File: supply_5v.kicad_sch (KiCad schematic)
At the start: 13 parts, among them IC2 TPS564242DRLR

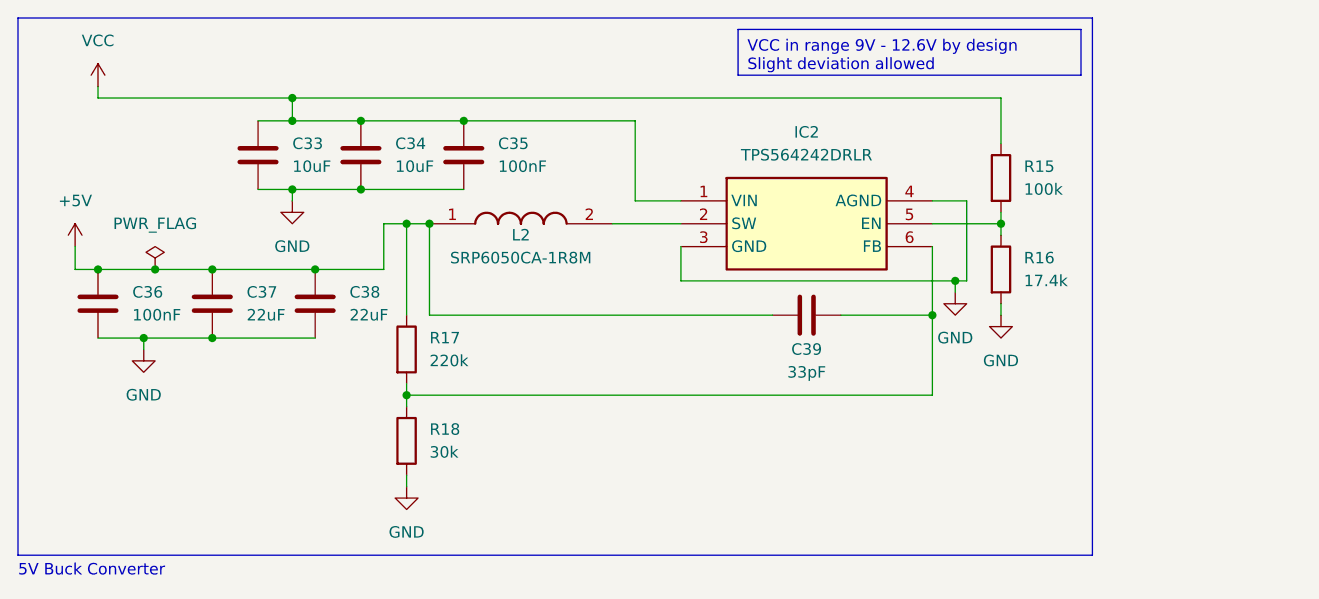
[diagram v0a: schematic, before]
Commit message: Uploaded all project files, finished PCB design
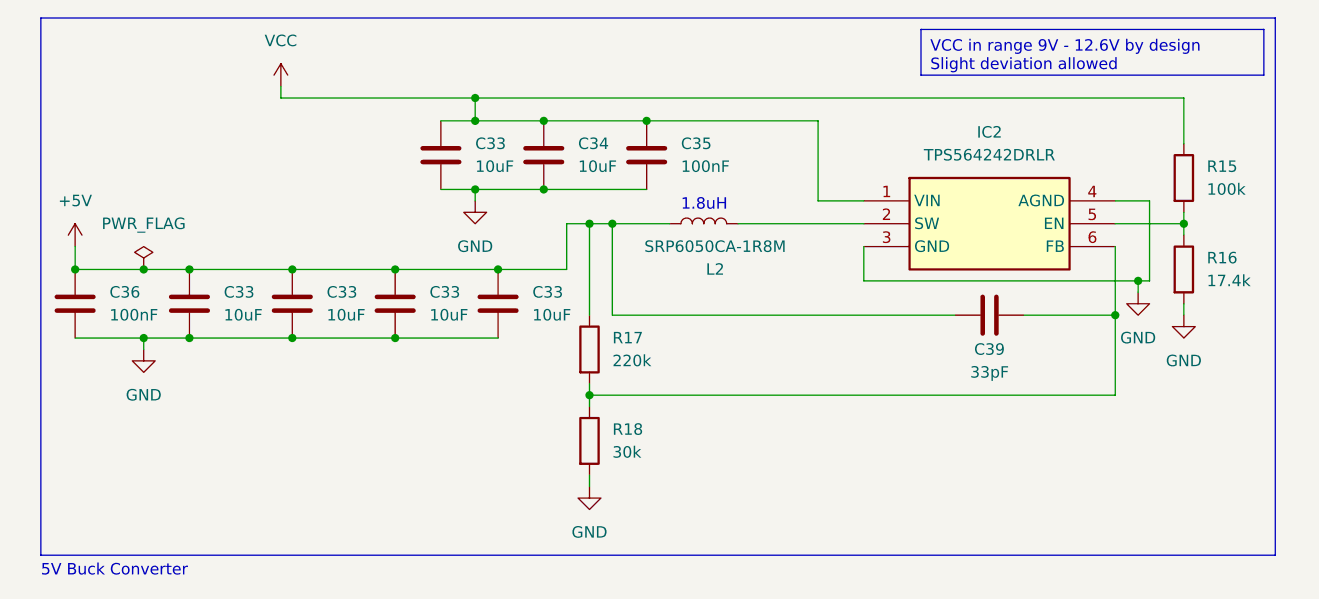
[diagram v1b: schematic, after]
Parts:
- removed C37, C38: 22uF, Capacitor_SMD:C_0805_2012Metric, symbol Device:C
- added C33 (x4): 10uF, Capacitor_SMD:C_0805_2012Metric, symbol Device:C
- L2: symbol parts:SRP6050CA-1R8M -> Device:L
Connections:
- net +5V: now also C33.1, C33.1, C33.1, C33.1
- net GND: now also C33.2, C33.2, C33.2, C33.2
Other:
- note added: "1.8uH"
- moved on the sheet: C33, C34, C35, C36, C39, IC2, R15, R16, R17, R18
